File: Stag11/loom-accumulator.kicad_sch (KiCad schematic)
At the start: 43 parts, among them J3 Conn_01x12, J4 Conn_01x12, J5 ATM064S, J6 ATM064S, J7 ATM064S, M1 AIL FAN

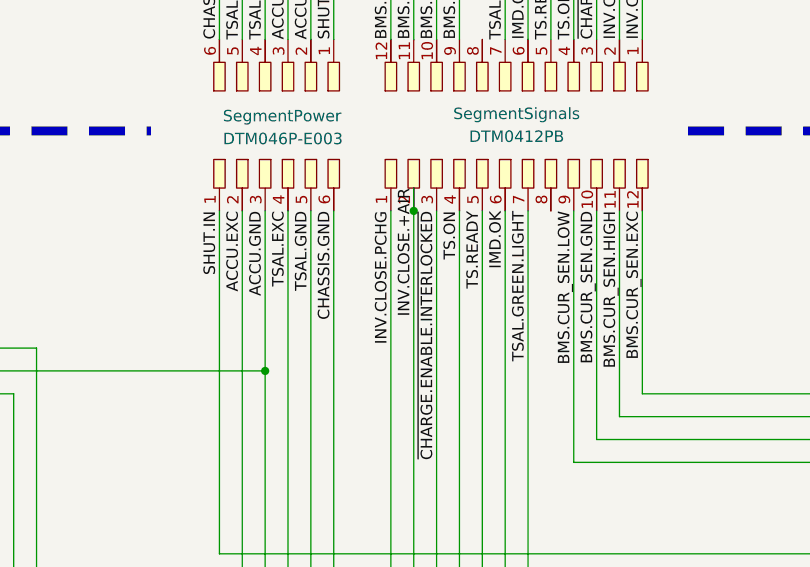
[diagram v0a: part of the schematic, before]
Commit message: updates
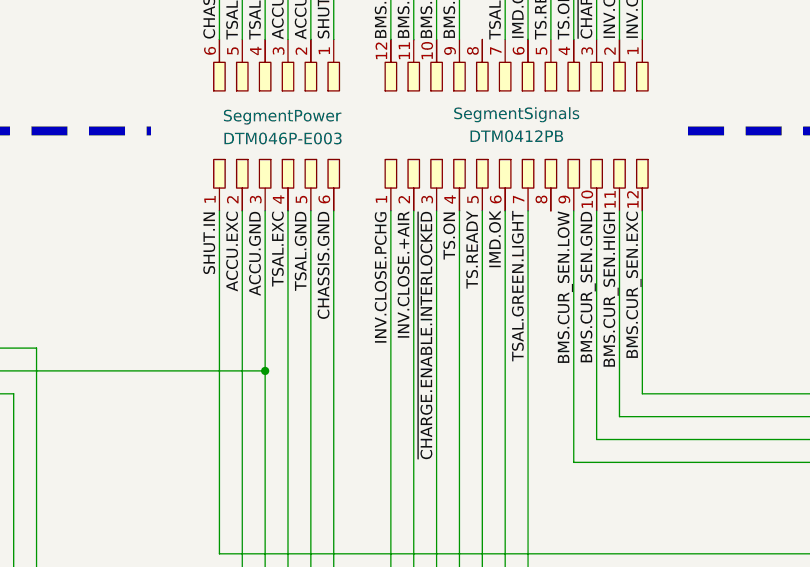
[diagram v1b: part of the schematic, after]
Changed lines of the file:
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@@
 	)
 	(junction
-		(at 154.94 205.74)
-		(diameter 0)
-		(color 0 0 0 0)
-	)
-	(junction
 		(at 138.43 318.77)
 		(diameter 0)
@@
 	(wire
 		(pts
-			(xy 154.94 203.2) (xy 154.94 205.74)
-		)
-		(stroke
-			(width 0)
-			(type default)
-		)
-	)
-	(wire
-		(pts
 			(xy 68.58 88.9) (xy 125.73 88.9)
 		)
@@
 	)
 	(label "INV.CLOSE.+AIR"
-		(at 154.94 203.2 270)
+		(at 154.94 205.74 270)
 		(fields_autoplaced yes)
 		(effects
